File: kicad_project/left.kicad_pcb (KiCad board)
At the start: 2 copper layers, 128.1 x 118.1 mm, 74 parts

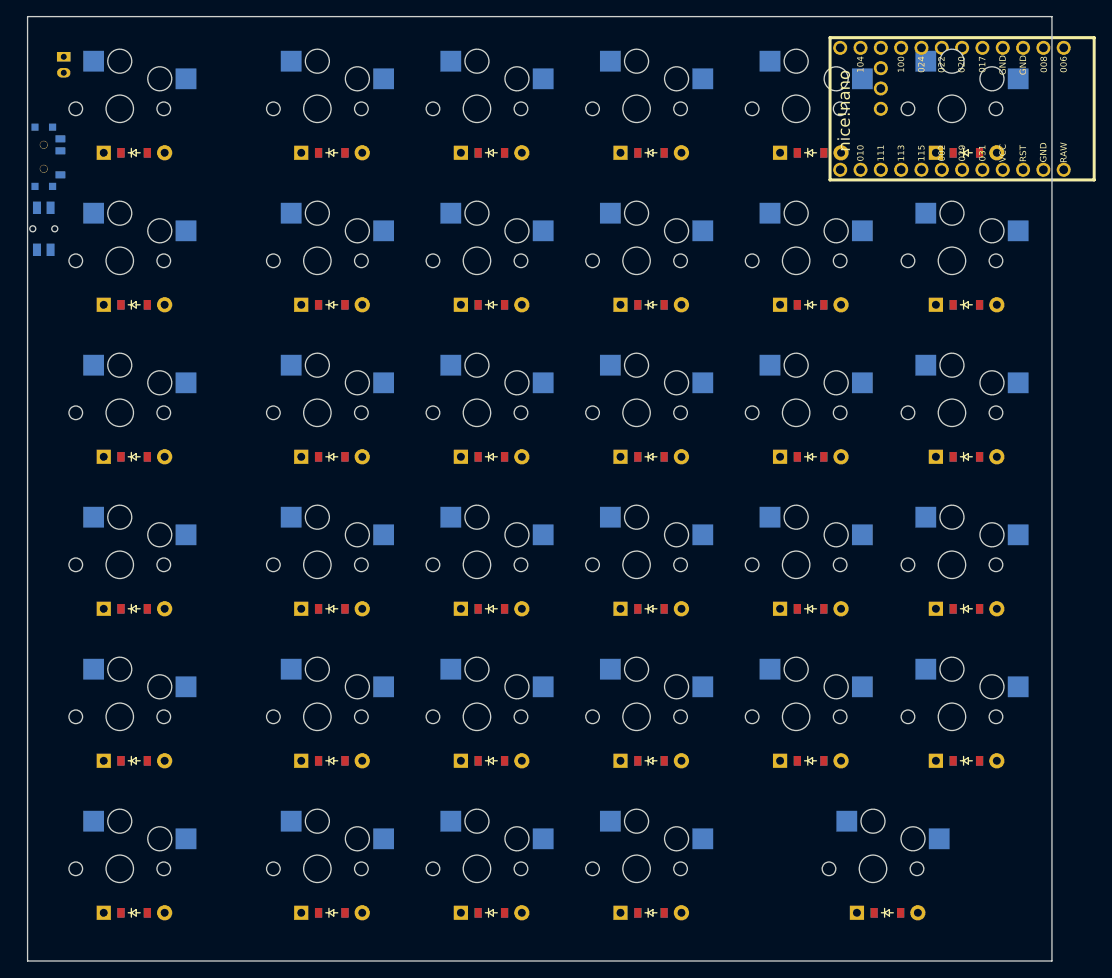
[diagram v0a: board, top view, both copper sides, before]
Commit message: please
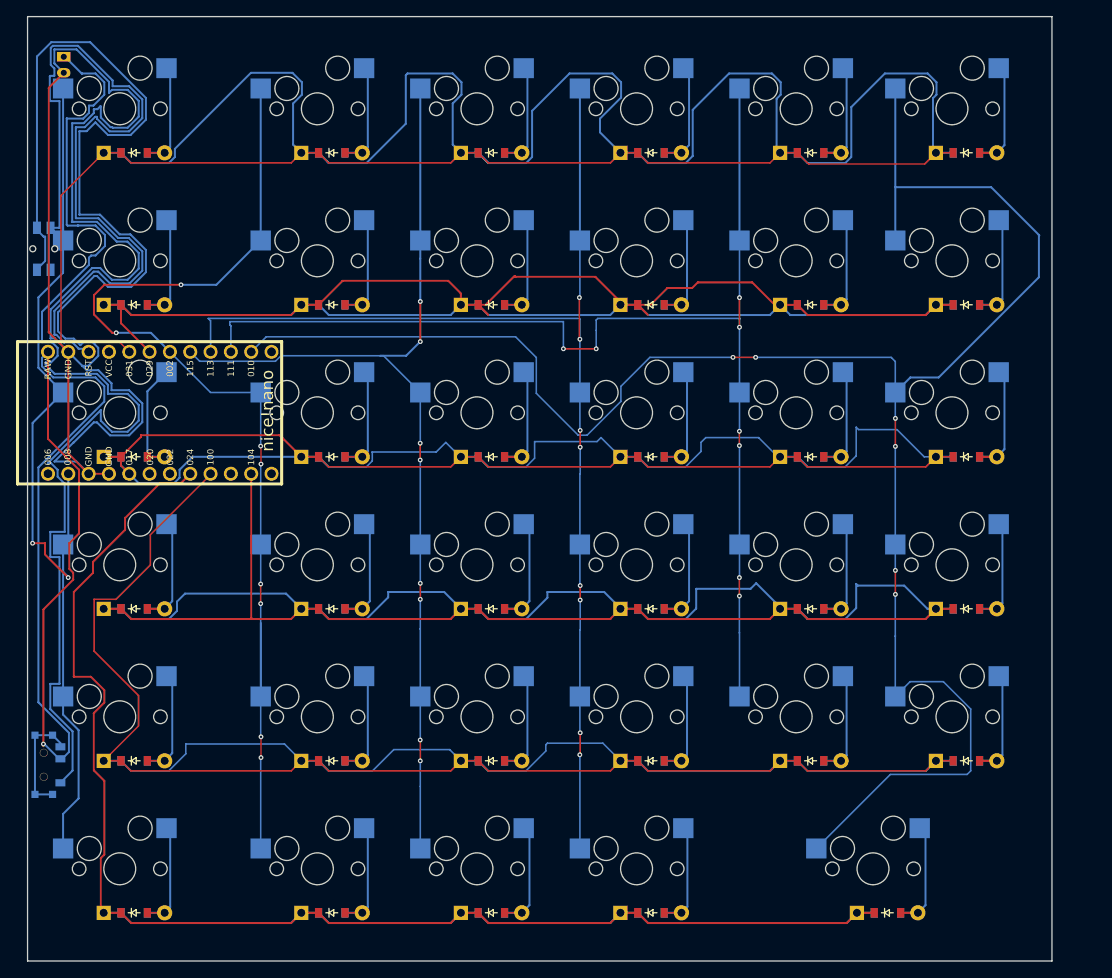
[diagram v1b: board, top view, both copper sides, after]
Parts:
- S1, S10, S11, S12, S13, S14, S15, S16, S17, S18, S19, S2, S20, S21, S22, S23, S24, S25, S26, S27, S28, S29, S3, S30, S31, S32, S33, S34, S35, S4, S5, S6, S7, S8, S9: footprint PG1350 -> MX
- moved MCU1 106.1 mm to (110.8, 143.0), turned to 0 degrees
- moved T1 76.0 mm to (96.3, 187.0)
- moved B1 2.50 mm to (96.3, 122.5)
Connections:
- D1 pad 1: P113 -> P024
- D10 pad 1: P029 -> P017
- D11 pad 1: P031 -> P029
- D12 pad 1: P006 -> P031
- D13 pad 1: P113 -> P024
- D14 pad 1: P115 -> P100
- D15 pad 1: P002 -> P104
- D16 pad 1: P029 -> P017
- D17 pad 1: P031 -> P029
- D18 pad 1: P006 -> P031
- D19 pad 1: P113 -> P024
- D2 pad 1: P115 -> P100
- D20 pad 1: P115 -> P100
- D21 pad 1: P002 -> P104
- D22 pad 1: P029 -> P017
- D23 pad 1: P031 -> P029
- D24 pad 1: P006 -> P031
- D25 pad 1: P115 -> P100
- D26 pad 1: P002 -> P104
- D27 pad 1: P029 -> P017
- D28 pad 1: P031 -> P029
- D29 pad 1: P006 -> P031
- D3 pad 1: P002 -> P104
- D30 pad 1: P115 -> P100
- D31 pad 1: P002 -> P104
- D32 pad 1: P029 -> P017
- D33 pad 1: P031 -> P029
- D34 pad 1: P006 -> P031
- D35 pad 1: P009 -> P024
- D4 pad 1: P029 -> P017
- D5 pad 1: P031 -> P029
- D6 pad 1: P006 -> P031
- D7 pad 1: P113 -> P024
- D8 pad 1: P115 -> P100
- D9 pad 1: P002 -> P104
- S1 pad 1: P020 -> P008
- S10 pad 1: P022 -> P002
- S11 pad 1: P022 -> P002
- S12 pad 1: P022 -> P002
- S13 pad 1: P024 -> P115
- S14 pad 1: P024 -> P115
- S15 pad 1: P024 -> P115
- S16 pad 1: P024 -> P115
- S17 pad 1: P024 -> P115
- S18 pad 1: P024 -> P115
- S19 pad 1: P100 -> P113
- S2 pad 1: P020 -> P008
- S20 pad 1: P100 -> P113
- S21 pad 1: P100 -> P113
- S22 pad 1: P100 -> P113
- S23 pad 1: P100 -> P113
- S24 pad 1: P100 -> P113
- S25 pad 1: P011 -> P111
- S26 pad 1: P011 -> P111
- S27 pad 1: P011 -> P111
- S28 pad 1: P011 -> P111
- S29 pad 1: P011 -> P111
- S3 pad 1: P020 -> P008
- S30 pad 1: P017 -> P010
- S31 pad 1: P017 -> P010
- S32 pad 1: P017 -> P010
- S33 pad 1: P017 -> P010
- S34 pad 1: P017 -> P010
- S35 pad 1: (no net) -> P010
- S4 pad 1: P020 -> P008
- S5 pad 1: P020 -> P008
- S6 pad 1: P020 -> P008
- S7 pad 1: P022 -> P002
- S8 pad 1: P022 -> P002
- S9 pad 1: P022 -> P002
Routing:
- net P031: track 0.00 -> 346.8 mm
- net P100: track 0.00 -> 279.9 mm
- net GND: track 0.00 -> 274.2 mm
- net P024: track 0.00 -> 267.8 mm
- net P104: track 0.00 -> 256.3 mm
- net P017: track 0.00 -> 250.0 mm
- net P010: track 0.00 -> 248.7 mm, vias 0 -> 6
- net P029: track 0.00 -> 241.8 mm
- net P111: track 0.00 -> 152.0 mm, vias 0 -> 8
- net P113: track 0.00 -> 148.5 mm, vias 0 -> 8
- net P002: track 0.00 -> 136.4 mm, vias 0 -> 8
- net pos: track 0.00 -> 135.3 mm
- net P115: track 0.00 -> 126.0 mm, vias 0 -> 8
- net P008: track 0.00 -> 124.9 mm, vias 0 -> 2
- net RAW: track 0.00 -> 119.1 mm, vias 0 -> 1
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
